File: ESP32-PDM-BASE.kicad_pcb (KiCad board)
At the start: 2 copper layers, 102.9 x 74.2 mm, 80 parts, among them J1 Conn_02x06_Top_Bottom, J3 USB4145-03-0170-C, J4 Conn_01x04, J5 Conn_02x05_Top_Bottom, Q1 BC817-25LT1G, Q2 BC817-25LT1G, Q3 BC817-25LT1G, Q4 BC817-25LT1G, Q5 BC817-25LT1G, Q6 BC817-25LT1G, U1 ESP32-S3-MINI-1, U3 LMR51610YDBVR, U4 CH340C, U5 ISO1044, U6 TPS7B91050, U7 LTV-247

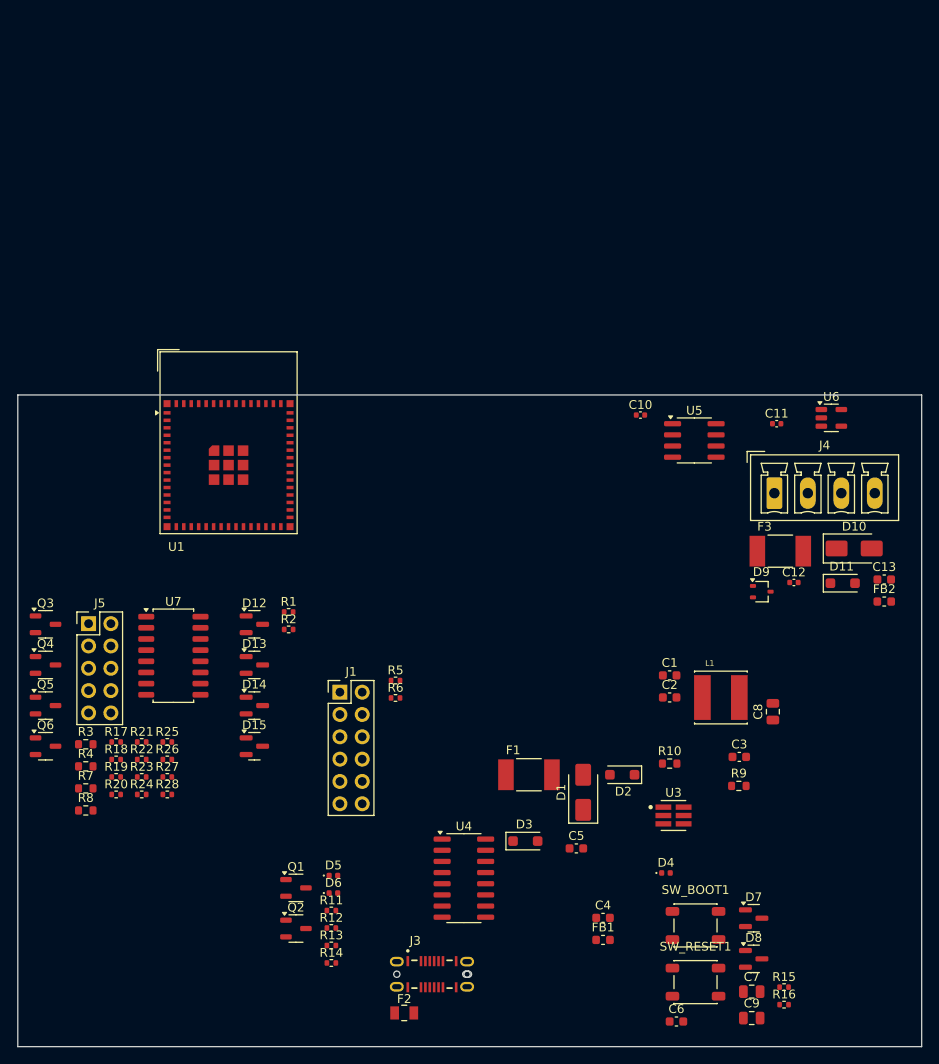
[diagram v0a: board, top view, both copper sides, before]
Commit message: unfinished work
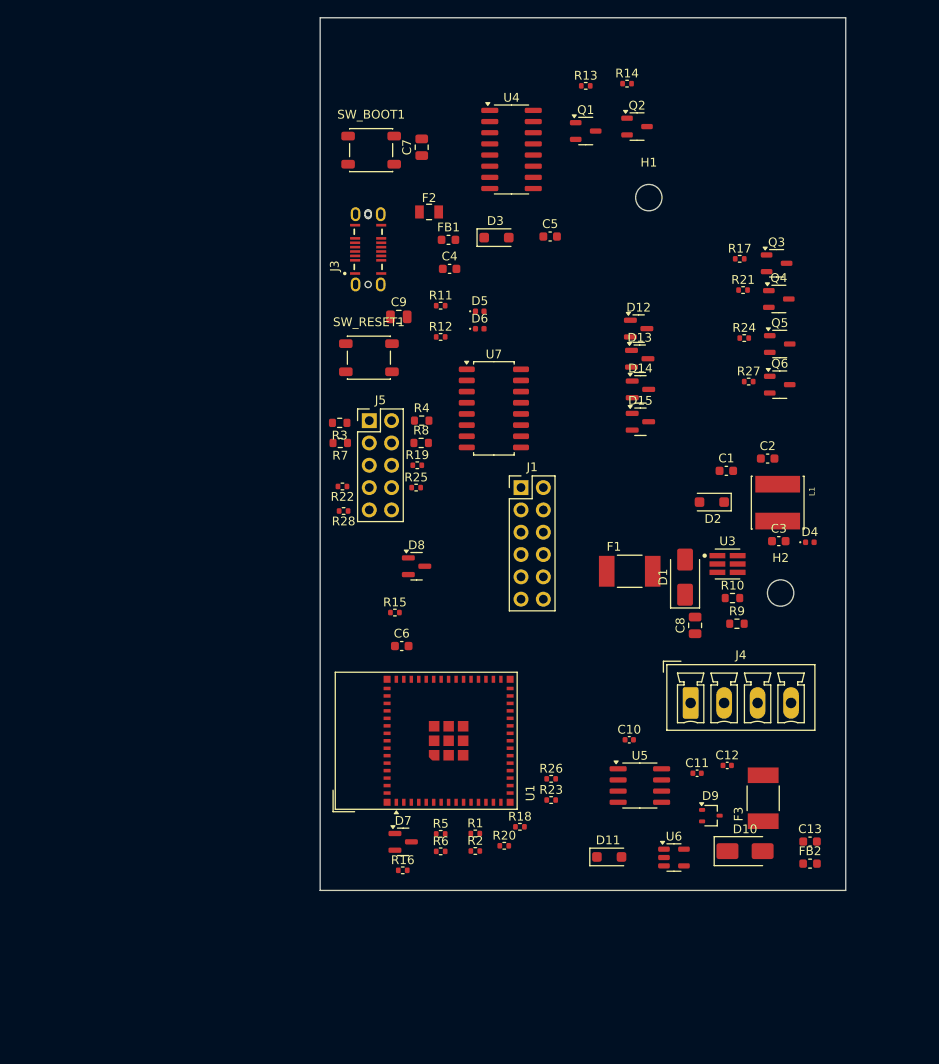
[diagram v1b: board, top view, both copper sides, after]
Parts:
- added H1: MountingHole, MountingHole:MountingHole_3mm, F.Cu at (149.5, 62.9)
- added H2: MountingHole, MountingHole:MountingHole_3mm, F.Cu at (164.5, 107.9)
- moved R14 105.6 mm to (147.1, 49.9)
- moved C7 103.2 mm to (123.7, 57.1), turned to 90 degrees
- moved R13 102.0 mm to (142.4, 50.2)
- moved Q2 99.2 mm to (148.2, 54.8)
- moved SW_BOOT1 95.7 mm to (117.9, 57.5)
- moved Q4 93.3 mm to (164.3, 74.4)
- moved Q5 93.1 mm to (164.4, 79.5)
- moved Q6 93.1 mm to (164.4, 84.2)
- moved Q3 92.8 mm to (164.1, 70.4)
- moved Q1 92.2 mm to (142.4, 55.3)
- moved F2 91.2 mm to (124.5, 64.5)
- moved R17 89.8 mm to (159.9, 69.8)
- moved C9 89.3 mm to (121.1, 76.5)
- moved R24 86.0 mm to (160.4, 78.9)
- moved R21 85.6 mm to (160.3, 73.4)
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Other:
- board size 102.9 x 74.2 mm -> 59.8 x 99.3 mm
